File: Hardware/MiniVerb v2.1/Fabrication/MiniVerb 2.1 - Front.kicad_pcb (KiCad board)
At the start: 2 copper layers, 47.9 x 128.5 mm, 48 parts, among them J1 IDC_2x05, U1 TL074, U2 LM4040DBZ-10, U3 MCP6001-OT

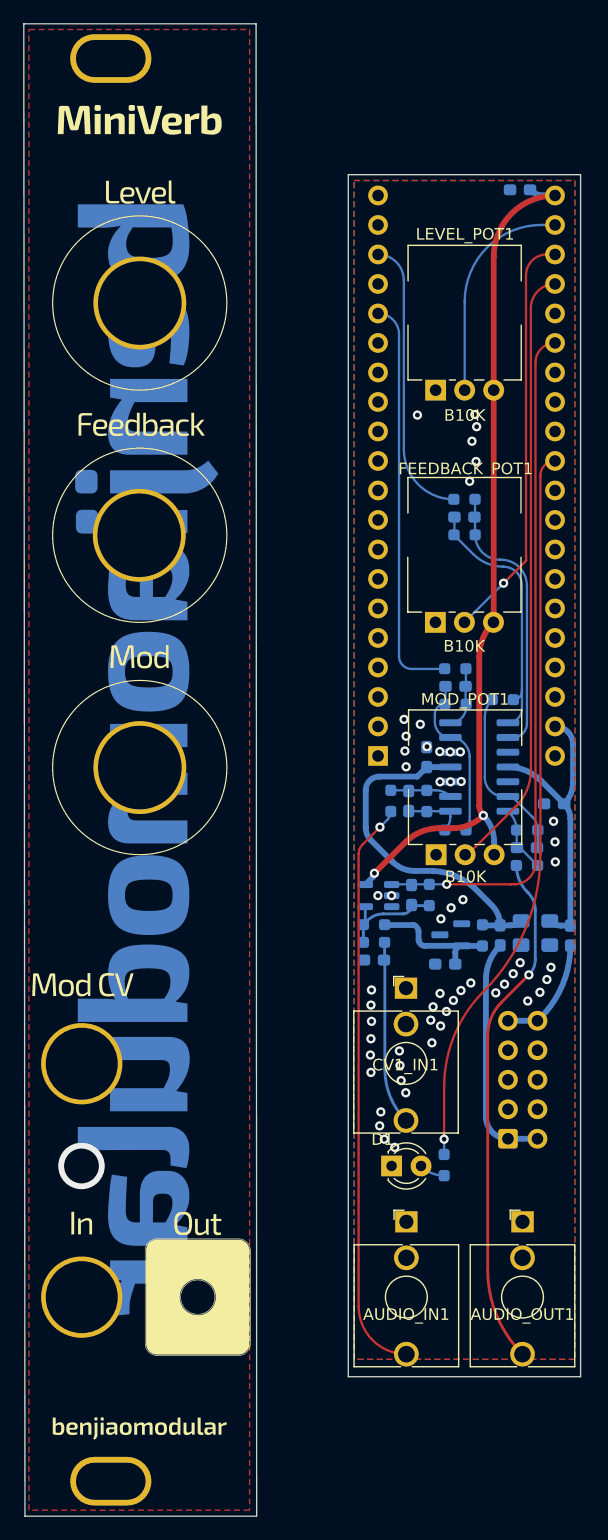
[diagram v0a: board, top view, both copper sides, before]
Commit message: Cleanup
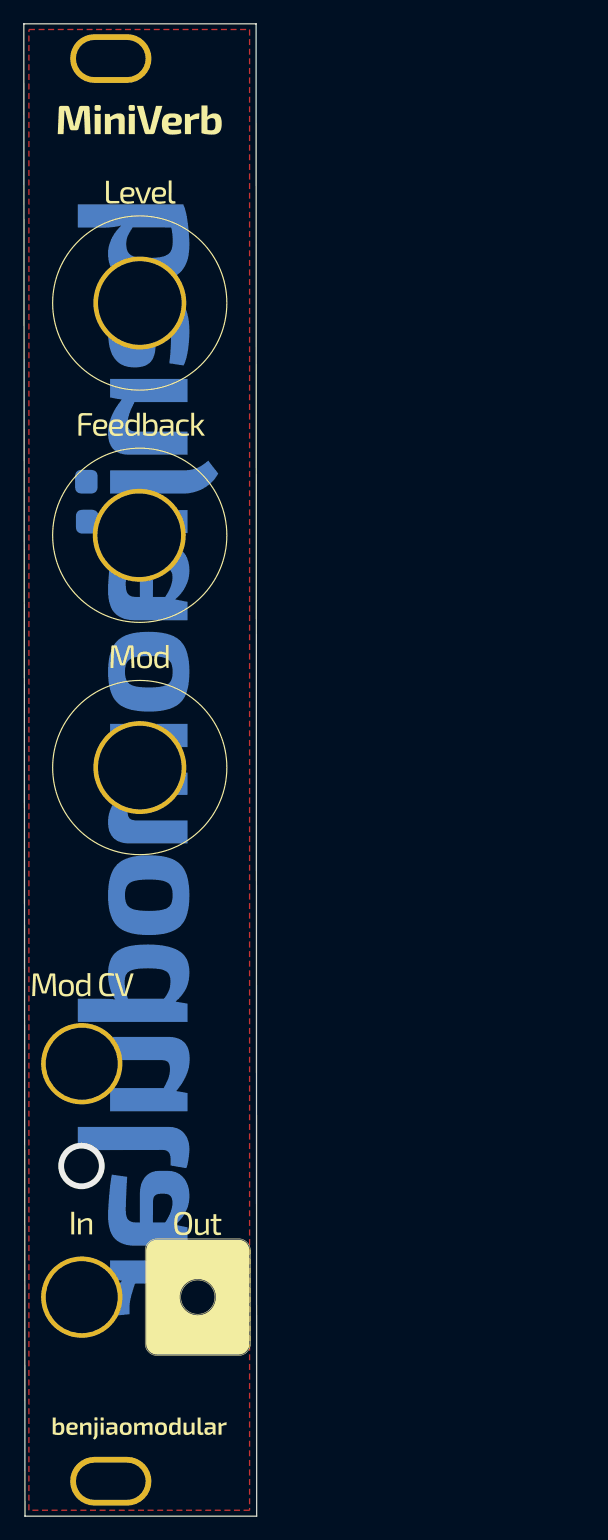
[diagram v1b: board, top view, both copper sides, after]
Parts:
- removed A1: Device_Audio_Electrosmith_Daisy_Seed_Rev4, daisy-seed:Device_Audio_Electrosmith_Daisy_Seed
- removed AUDIO_IN1, AUDIO_OUT1, CV1_IN1: MONO_JACK, benjiaomodular:AudioJack_3.5mm
- removed C1, C2, C4: 47pF, Capacitor_SMD:C_0603_1608Metric_Pad1.08x0.95mm_HandSolder
- removed C10, C13, C7, C8, C9: 100nF, Capacitor_SMD:C_0603_1608Metric_Pad1.08x0.95mm_HandSolder
- removed C14: 10nF, Capacitor_SMD:C_0603_1608Metric_Pad1.08x0.95mm_HandSolder
- removed C3: 680pF, Capacitor_SMD:C_0603_1608Metric_Pad1.08x0.95mm_HandSolder
- removed C5, C6: 47uF, Capacitor_SMD:C_0805_2012Metric_Pad1.18x1.45mm_HandSolder
- removed D1: 3mm_LED, LED_THT:LED_D3.0mm
- removed FB1, FB2: 742792664, Capacitor_SMD:C_0603_1608Metric_Pad1.08x0.95mm_HandSolder
- removed FEEDBACK_POT1, LEVEL_POT1, MOD_POT1: B10K, benjiaomodular:Potentiometer_RV09_NoBracket
- removed J1: IDC_2x05, Connector_IDC:IDC-Header_2x05_P2.54mm_Vertical
- removed R1, R7: 10k, Resistor_SMD:R_0603_1608Metric_Pad0.98x0.95mm_HandSolder
- removed R10, R9: 1k, Resistor_SMD:R_0603_1608Metric_Pad0.98x0.95mm_HandSolder
- removed R11: 220, Resistor_SMD:R_0603_1608Metric_Pad0.98x0.95mm_HandSolder
- removed R12: 330, Resistor_SMD:R_0603_1608Metric_Pad0.98x0.95mm_HandSolder
- removed R13: 200k, Resistor_SMD:R_0603_1608Metric_Pad0.98x0.95mm_HandSolder
- removed R16, R2, R3, R4, R5, R6, R8: 100k, Resistor_SMD:R_0603_1608Metric_Pad0.98x0.95mm_HandSolder
- removed R17: 66.5k, Resistor_SMD:R_0603_1608Metric_Pad0.98x0.95mm_HandSolder
- removed U1: TL074, Package_SO:SOIC-14_3.9x8.7mm_P1.27mm
- removed U2: LM4040DBZ-10, Package_TO_SOT_SMD:SOT-23
- removed U3: MCP6001-OT, Package_TO_SOT_SMD:SOT-23-5
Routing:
- net 3V3_A: track 74.8 -> 0.00 mm, vias 2 -> 0
- net LED: track 62.5 -> 0.00 mm, vias 1 -> 0
- net CV1: track 59.0 -> 0.00 mm, vias 1 -> 0
- net MOD: track 52.5 -> 0.00 mm
- net Net-(AUDIO_IN1-PadT): track 50.0 -> 0.00 mm, vias 1 -> 0
- net Net-(AUDIO_OUT1-PadT): track 44.7 -> 0.00 mm, vias 1 -> 0
- net FEEDBACK: track 35.5 -> 0.00 mm, vias 1 -> 0
- net INT_AUDIO_IN1: track 35.0 -> 0.00 mm
- net -12V: track 30.4 -> 0.00 mm
- net +12V: track 26.1 -> 0.00 mm
- net INT_AUDIO_OUT1: track 24.5 -> 0.00 mm
- net Net-(C1-Pad2): track 24.0 -> 0.00 mm
- net Net-(C1-Pad1): track 22.9 -> 0.00 mm
- net Net-(FB2-Pad1): track 20.5 -> 0.00 mm
- net LEVEL: track 18.9 -> 0.00 mm
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- removed copper zone on B.Cu, net GND
- removed copper zone on F.Cu, net GND
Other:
- board size 47.9 x 128.5 mm -> 20.1 x 128.5 mm
